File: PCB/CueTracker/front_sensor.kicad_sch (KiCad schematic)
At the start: 38 parts, among them J201 FH34SRJ-24S-0.5SH(50), U11 IIS3DWB10ISTR, U12 LSM6DSV320XTR, U15 TPS22919, U6 BMP581, U8 MMC5983MA

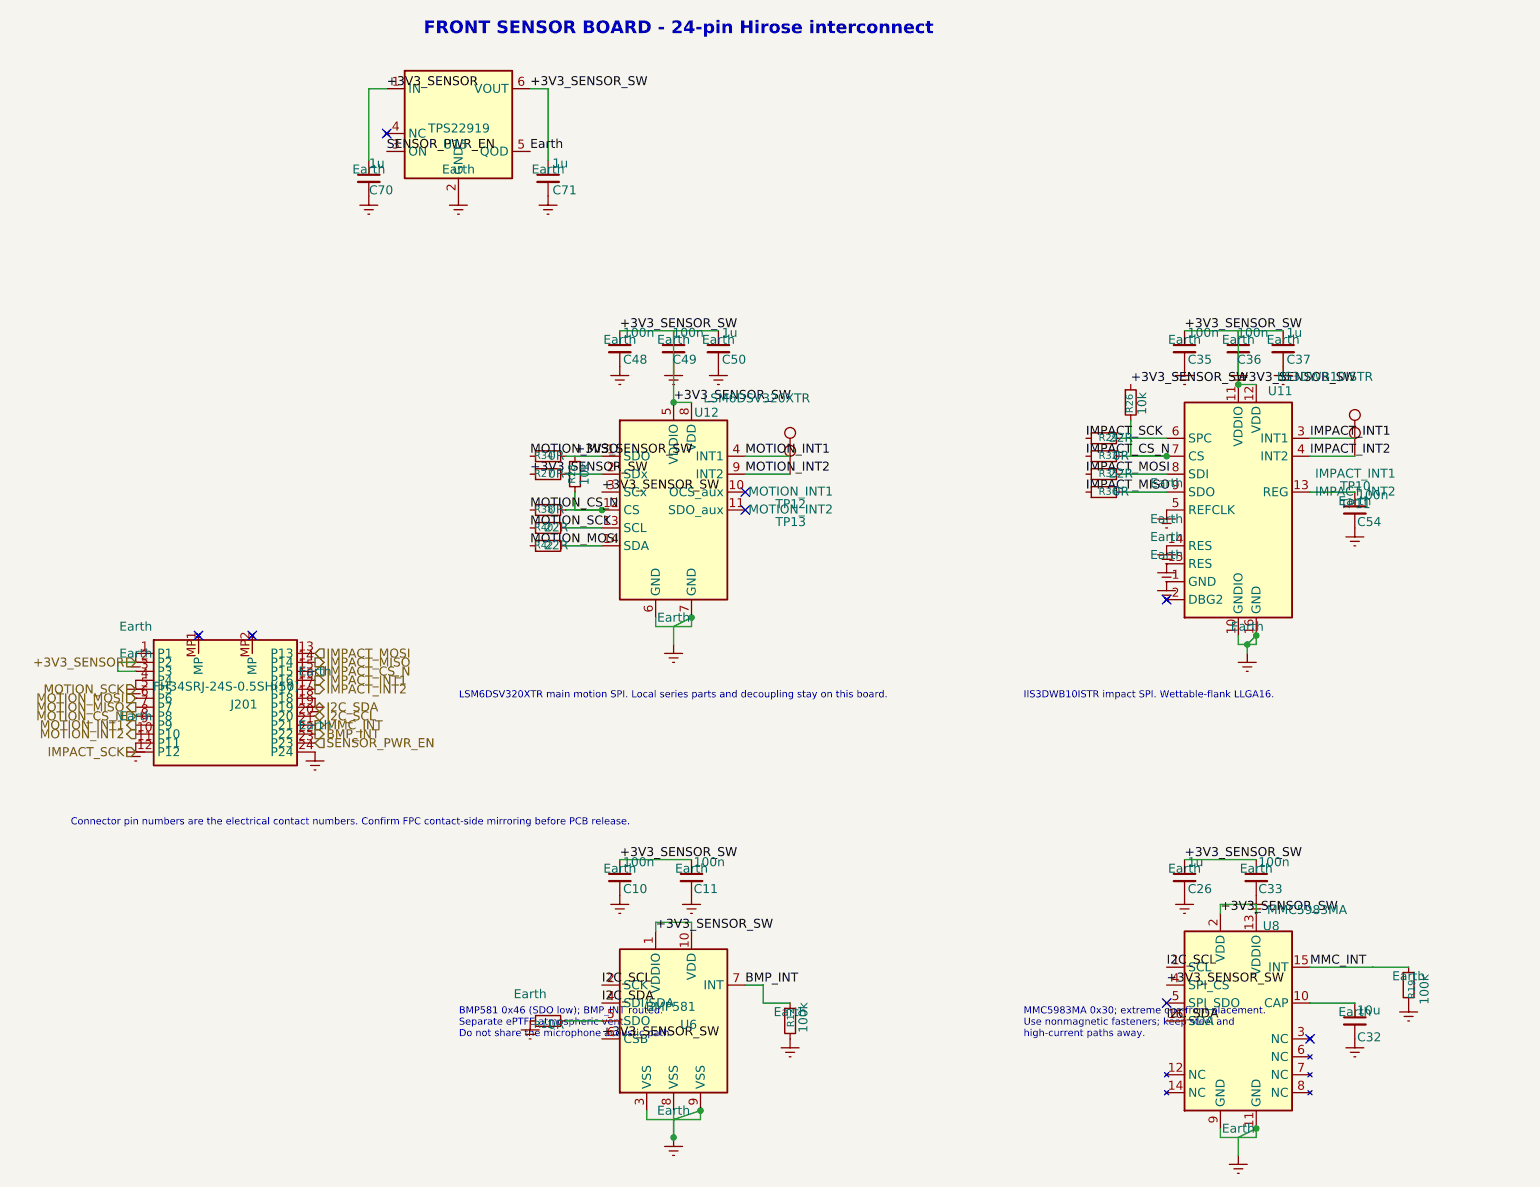
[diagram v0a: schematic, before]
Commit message: pcb: clean up CueTracker split
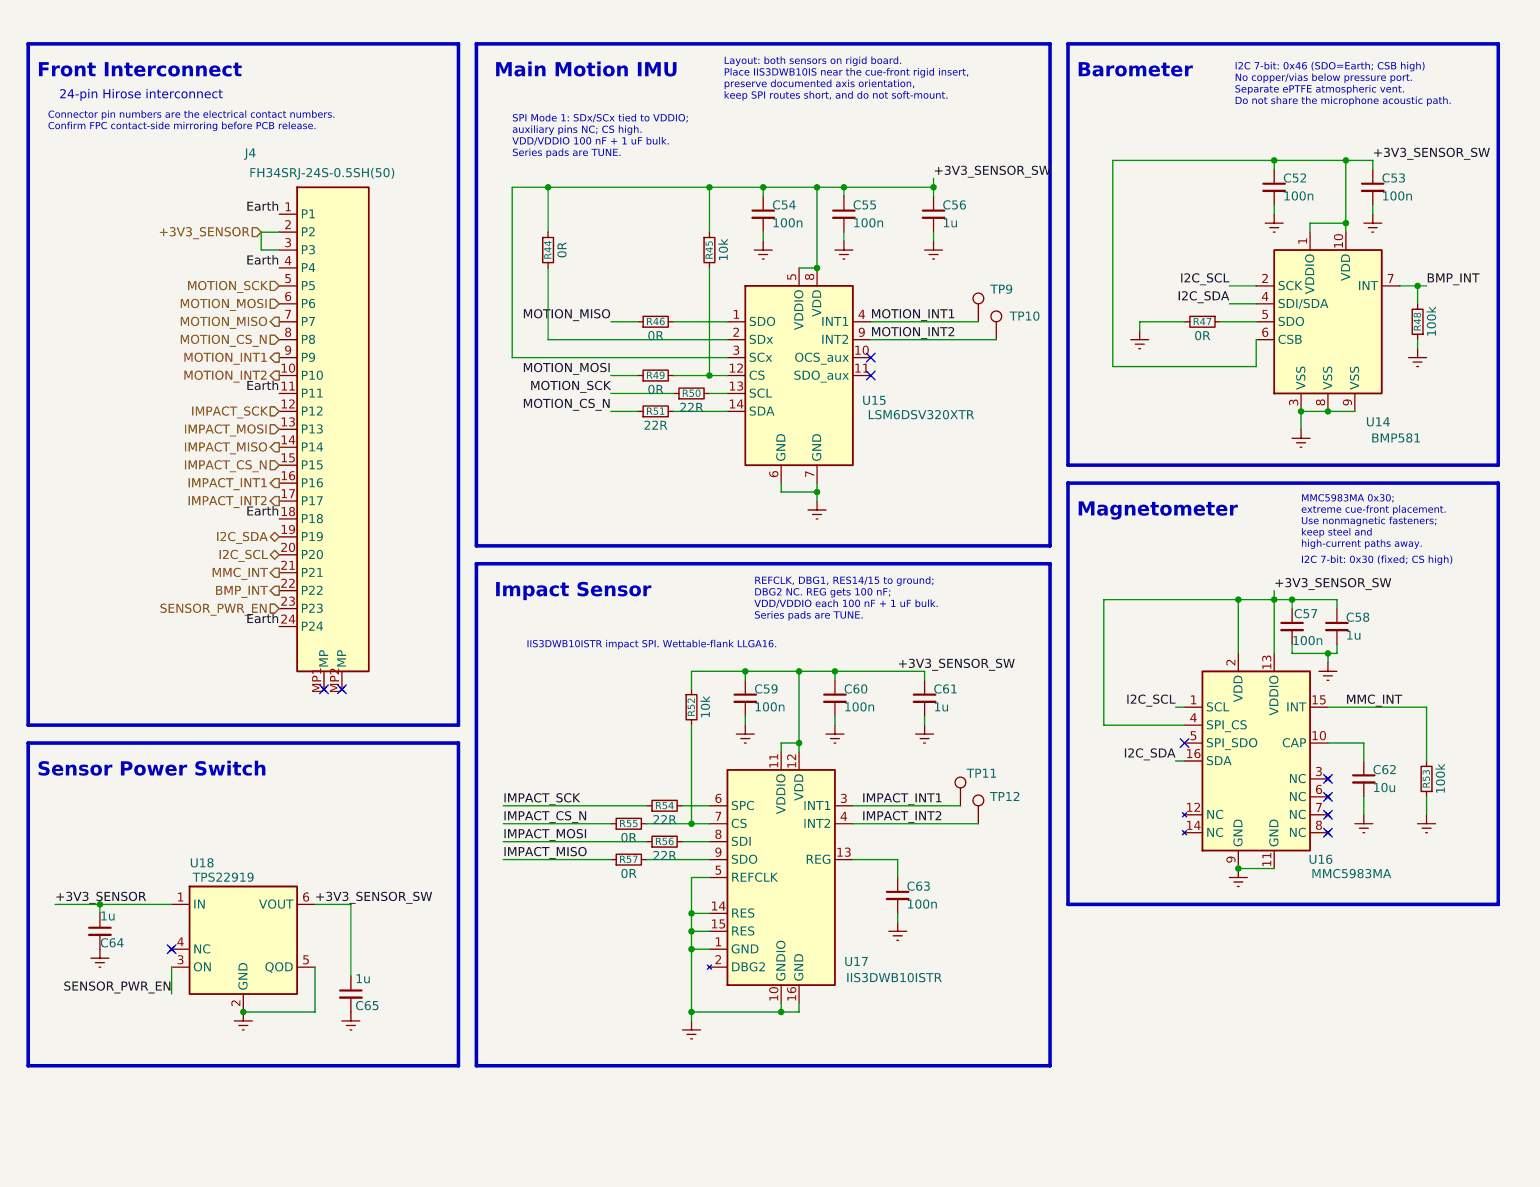
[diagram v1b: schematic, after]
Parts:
- removed C10, C11, C33, C35, C36, C48, C49: 100n, Capacitor_SMD:C_0603_1608Metric, symbol Device:C_Small
- removed C26, C37, C50: 1u, Capacitor_SMD:C_0603_1608Metric, symbol Device:C_Small
- removed C32: 10u, Capacitor_SMD:C_0805_2012Metric, symbol Device:C_Small
- removed R11, R27, R32, R34, R36, R38: 0R, Resistor_SMD:R_0603_1608Metric, symbol Device:R_Small
- removed R12, R19: 100k, Resistor_SMD:R_0603_1608Metric, symbol Device:R_Small
- removed R26, R28: 10k, Resistor_SMD:R_0603_1608Metric, symbol Device:R_Small
- removed R29, R35, R40, R42: 22R, Resistor_SMD:R_0603_1608Metric, symbol Device:R_Small
- removed TP13: MOTION_INT2, TestPoint:TestPoint_Pad_D1.0mm, symbol Connector:TestPoint
- removed U11: IIS3DWB10ISTR, CueTracker_Exact:IIS3DWB10IS_LLGA16_4.5x4.5_WF, symbol CueTracker_Exact:IIS3DWB10ISTR
- removed U12: LSM6DSV320XTR, Package_LGA:LGA-14_3x2.5mm_P0.5mm_LayoutBorder3x4y, symbol CueTracker_Exact:LSM6DSV320XTR
- removed U6: BMP581, CueTracker_Exact:BMP581_LGA10_2x2mm, symbol CueTracker_Exact:BMP581
- removed U8: MMC5983MA, CueTracker_Exact:MMC5983MA_LGA16_3x3mm, symbol CueTracker_Exact:MMC5983MA
- added C52, C53, C55, C59, C60, C63: 100n, Capacitor_SMD:C_0402_1005Metric, symbol Device:C_Small
- added C56, C58, C61: 1u, Capacitor_SMD:C_0402_1005Metric, symbol Device:C_Small
- added C57: 100n, Capacitor_SMD:C_0603_1608Metric, symbol Device:C_Small
- added C62: 10u, Capacitor_SMD:C_0603_1608Metric, symbol Device:C_Small
- added R44, R46, R47, R49, R55, R57: 0R, Resistor_SMD:R_0402_1005Metric, symbol Device:R_Small
- added R45, R52: 10k, Resistor_SMD:R_0402_1005Metric, symbol Device:R_Small
- added R48, R53: 100k, Resistor_SMD:R_0402_1005Metric, symbol Device:R_Small
- added R50, R51, R54, R56: 22R, Resistor_SMD:R_0402_1005Metric, symbol Device:R_Small
- added TP9: MOTION_INT1, TestPoint:TestPoint_Pad_D1.0mm, symbol Connector:TestPoint
- added U14: BMP581, CueTracker_Exact:BMP581_LGA10_2x2mm, symbol CueTracker_Exact:BMP581
- added U15: LSM6DSV320XTR, Package_LGA:LGA-14_3x2.5mm_P0.5mm_LayoutBorder3x4y, symbol CueTracker_Exact:LSM6DSV320XTR
- added U16: MMC5983MA, CueTracker_Exact:MMC5983MA_LGA16_3x3mm, symbol CueTracker_Exact:MMC5983MA
- added U17: IIS3DWB10ISTR, CueTracker_Exact:IIS3DWB10IS_LLGA16_4.5x4.5_WF, symbol CueTracker_Exact:IIS3DWB10ISTR
- C54: footprint Capacitor_SMD:C_0603_1608Metric -> Capacitor_SMD:C_0402_1005Metric; Voltage 6.3 V min -> 10 V
- TP10: value IMPACT_INT1 -> MOTION_INT2; Population (none) -> Populate
- TP11: value IMPACT_INT2 -> IMPACT_INT1; Population (none) -> Populate
- TP12: value MOTION_INT1 -> IMPACT_INT2; Population (none) -> Populate
- renumbered C70 to C64, C71 to C65, J201 to J4, U15 to U18
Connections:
- net +3V3_SENSOR_SW: now also C54.1, C52.1, C53.1, C55.1, C56.1, C57.1, C58.1, C59.1, C60.1, C61.1, R44.1, R45.1, R52.1, U14.1 (VDDIO), U14.10 (VDD), U14.6 (CSB), U15.3 (SCx), U15.5 (VDDIO), U15.8 (VDD), U16.13 (VDDIO), U16.2 (VDD), U16.4 (SPI_CS), U17.11 (VDDIO), U17.12 (VDD)
- net BMP_INT: now also R48.2, U14.7 (INT)
- net Earth: now also C52.2, C53.2, C55.2, C56.2, C57.2, C58.2, C59.2, C60.2, C61.2, C62.2, C63.2, R47.2, R48.1, R53.1, U14.3 (VSS), U14.8 (VSS), U14.9 (VSS), U15.6 (GND), U15.7 (GND), U16.11 (GND), U16.9 (GND), U17.1 (GND), U17.10 (GNDIO), U17.14 (RES), U17.15 (RES), U17.16 (GND), U17.5 (REFCLK)
- net I2C_SCL: now also U14.2 (SCK), U16.1 (SCL)
- net I2C_SDA: now also U14.4 (SDI/SDA), U16.16 (SDA)
- net IMPACT_CS_N: now also R55.1
- net IMPACT_INT1: now also TP11.1, U17.3 (INT1); no longer TP10.1
- net IMPACT_INT2: now also TP12.1, U17.4 (INT2); no longer TP11.1
- net IMPACT_MISO: now also R57.1
- net IMPACT_MOSI: now also R56.1
- net IMPACT_SCK: now also R54.1
- net MMC_INT: now also R53.2, U16.15 (INT)
- net MOTION_CS_N: now also R51.1
- net MOTION_INT1: now also TP9.1, U15.4 (INT1); no longer TP12.1
- net MOTION_INT2: now also TP10.1, U15.9 (INT2)
- net MOTION_MISO: now also R46.1
- net MOTION_MOSI: now also R49.1
- net MOTION_SCK: now also R50.1
- new net: R46.2, U15.1 (SDO)
- new net: R45.2, R49.2, U15.12 (CS)
- new net: R50.2, U15.13 (SCL)
- new net: R51.2, U15.14 (SDA)
- new net: R44.2, U15.2 (SDx)
- new net: R54.2, U17.6 (SPC)
- new net: R47.1, U14.5 (SDO)
- new net: C62.1, U16.10 (CAP)
- new net: R52.2, R55.2, U17.7 (CS)
- new net: C63.1, U17.13 (REG)
- new net: R56.2, U17.8 (SDI)
- new net: R57.2, U17.9 (SDO)
- no-connect marks 8 -> 10
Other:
- note added: "24-pin Hirose interconnect"
- note added: "Barometer"
- note added: "Front Interconnect"
- note added: "I2C 7-bit: 0x30 (fixed; CS high)"
- note added: "I2C 7-bit: 0x46 (SDO=Earth; CSB high) No copper/vias below pressure port. Separate ePTFE atmospheric vent. Do not share the microphone acoustic path."
- note added: "Impact Sensor"
- note added: "Layout: both sensors on rigid board. Place IIS3DWB10IS near the cue-front rigid insert, preserve documented axis orientation, keep SPI routes short, and do not soft-mount."
- note added: "Magnetometer"
- note added: "Main Motion IMU"
- note added: "REFCLK, DBG1, RES14/15 to ground; DBG2 NC. REG gets 100 nF; VDD/VDDIO each 100 nF + 1 uF bulk. Series pads are TUNE."
- note added: "SPI Mode 1: SDx/SCx tied to VDDIO; auxiliary pins NC; CS high. VDD/VDDIO 100 nF + 1 uF bulk. Series pads are TUNE."
- note added: "Sensor Power Switch"
- note removed: "BMP581 0x46 (SDO low); BMP_INT routed. Separate ePTFE atmospheric vent. Do not share the microphone acoustic path."
- note removed: "FRONT SENSOR BOARD - 24-pin Hirose interconnect"
- note removed: "LSM6DSV320XTR main motion SPI. Local series parts and decoupling stay on this board."
- moved on the sheet: C64, C65, J4, U18
